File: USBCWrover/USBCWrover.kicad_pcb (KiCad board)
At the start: 2 copper layers, 21 parts, among them J1 USB_C_Receptacle_USB2.0, Q1 Q_NMOS_GSD, Q2 Q_NMOS_GSD, SW1 SW_Push, SW2 SW_Push, U1 CH340C, U2 CP2104, U3 AMS1117-3.3

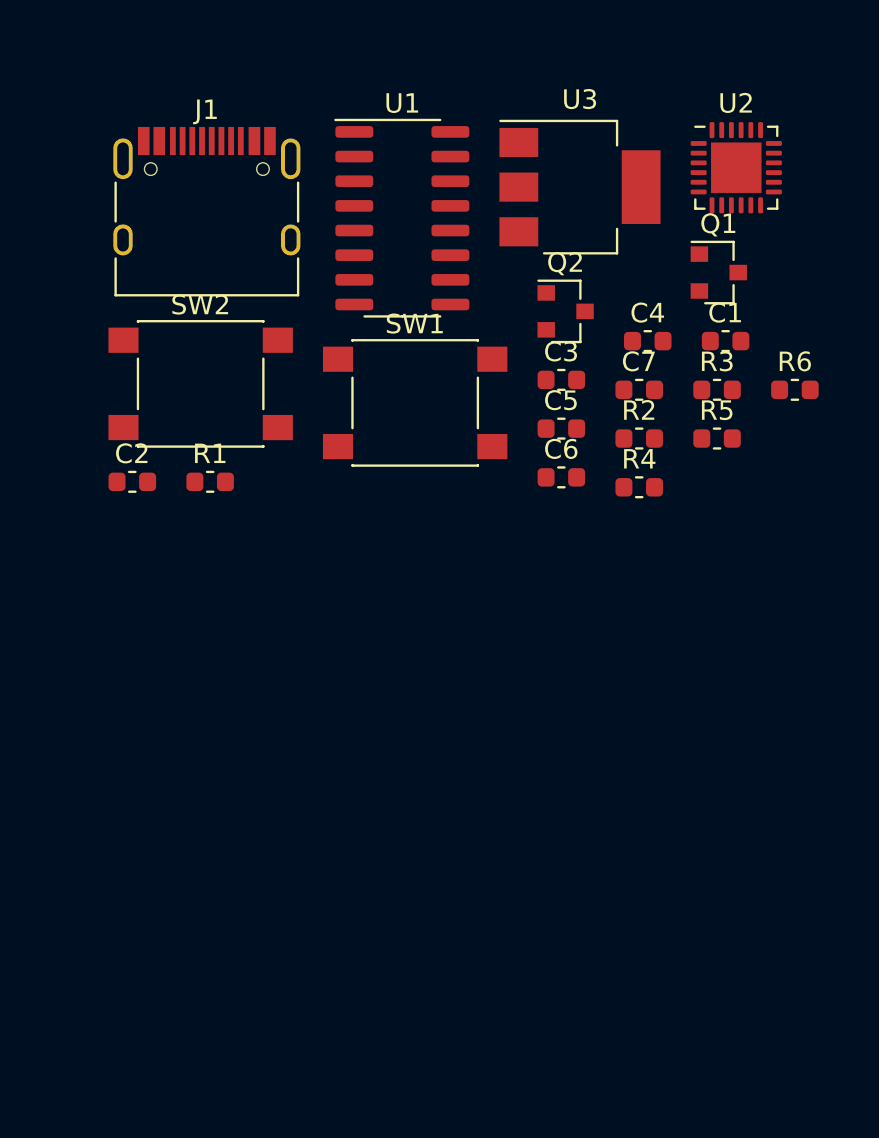
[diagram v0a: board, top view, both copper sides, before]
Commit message: routing done, but not pretty
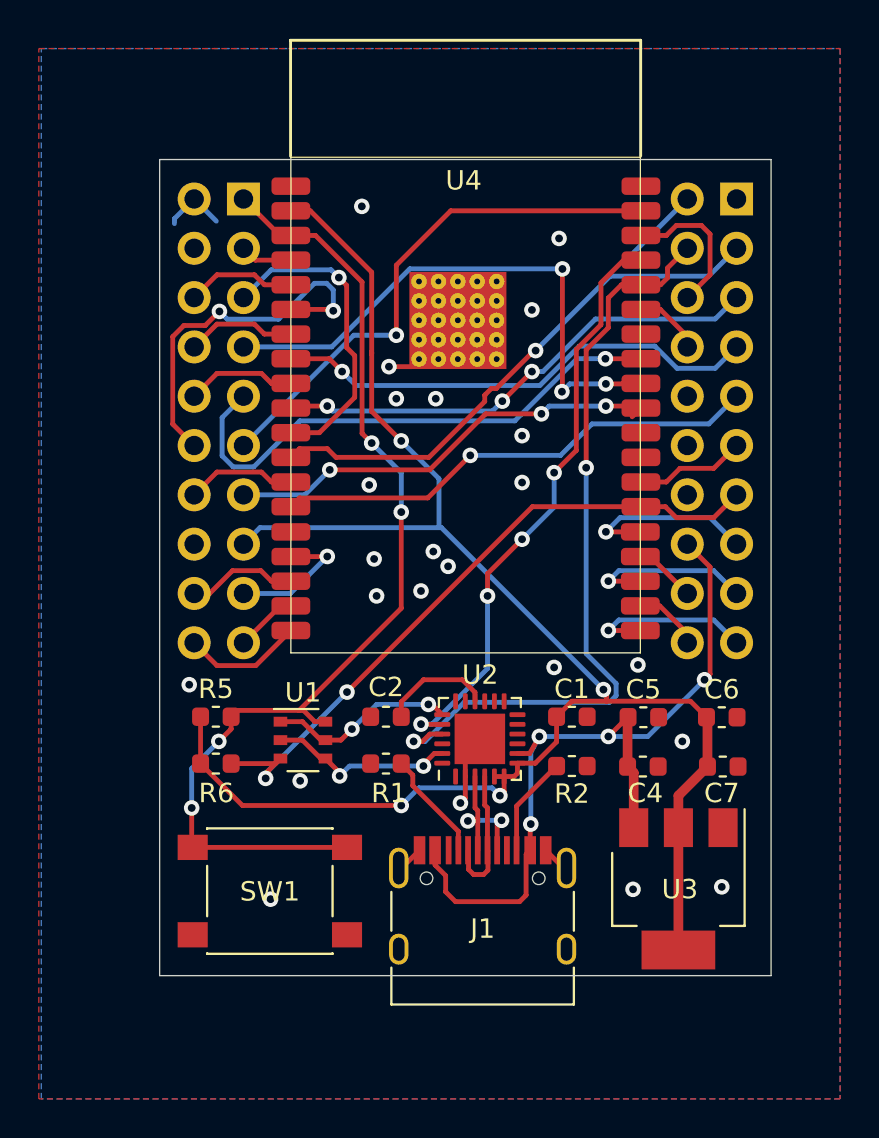
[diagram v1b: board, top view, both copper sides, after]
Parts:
- removed C3: 100nF, Capacitor_SMD:C_0603_1608Metric
- removed Q1, Q2: Q_NMOS_GSD, Package_TO_SOT_SMD:SOT-23
- removed R3, R4: 10k, Resistor_SMD:R_0603_1608Metric
- removed SW2: SW_Push, Button_Switch_SMD:SW_Push_1P1T_NO_6x6mm_H9.5mm
- added J2: Conn_02x10_Odd_Even, Connector_PinHeader_2.54mm:PinHeader_2x10_P2.54mm_Vertical, B.Cu at (154.9, 106.7)
- added J3: Conn_02x10_Odd_Even, Connector_PinHeader_2.54mm:PinHeader_2x10_P2.54mm_Vertical, B.Cu at (129.5, 106.7)
- added U4: ESP32-WROVER, esp32-wrover:ESP32-WROVER, F.Cu at (141.0, 105.1)
- U1: value CH340C -> UMH3N; footprint Package_SO:SOIC-16_3.9x9.9mm_P1.27mm -> Package_SO:TSOP-6_1.65x3.05mm_P0.95mm
- moved J1 39.2 mm to (141.9, 144.3)
- moved U3 36.5 mm to (151.9, 142.2), turned to 270 degrees
- moved R6 35.5 mm to (128.1, 135.8)
- moved U2 32.3 mm to (141.7, 134.5), turned to 90 degrees
- moved R5 29.5 mm to (128.1, 133.3)
- moved U1 27.4 mm to (132.6, 134.6)
- moved SW1 26.2 mm to (130.9, 142.3)
- moved C4 21.9 mm to (150.1, 135.9)
- moved C1 20.9 mm to (146.5, 133.3)
- moved C7 19.9 mm to (154.2, 135.9)
- moved C2 17.8 mm to (136.9, 133.3), turned to 180 degrees
- moved R2 17.2 mm to (146.5, 135.9), turned to 180 degrees
- moved R1 17.1 mm to (136.9, 135.8)
- moved C5 15.5 mm to (150.1, 133.4)
- moved C6 14.9 mm to (154.2, 133.4)
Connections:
- U1 pad 1: GND -> SER_RTS
- U1 pad 2: ESP_RXD -> SER_DTR
- U1 pad 3: ESP_TXD -> ESP_FLS
- U1 pad 4: Net-(U1-Pad4) -> SER_DTR
- U1 pad 5: USB_D+ -> SER_RTS
- U1 pad 6: USB_D- -> ESP_RST
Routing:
- net +3V3: track 0.00 -> 90.0 mm, vias 0 -> 4
- net ESP_RST: track 0.00 -> 53.7 mm, vias 0 -> 4
- net +5V: track 0.00 -> 41.4 mm, vias 0 -> 4
- net ESP_RXD: track 0.00 -> 40.1 mm, vias 0 -> 2
- net ESP_TXD: track 0.00 -> 35.0 mm, vias 0 -> 4
- net ESP_FLS: track 0.00 -> 34.9 mm, vias 0 -> 2
- net IO18: track 0.00 -> 29.6 mm, vias 0 -> 3
- net IO27: track 0.00 -> 28.0 mm, vias 0 -> 1
- net IO19: track 0.00 -> 27.6 mm, vias 0 -> 1
- net IO23: track 0.00 -> 27.6 mm, vias 0 -> 1
- net IO25: track 0.00 -> 25.5 mm, vias 0 -> 3
- net IO12: track 0.00 -> 25.3 mm, vias 0 -> 1
- net IO32: track 0.00 -> 25.3 mm, vias 0 -> 1
- net IO5: track 0.00 -> 23.0 mm, vias 0 -> 3
- net GND: track 0.00 -> 20.1 mm, vias 0 -> 23
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- added copper zone on B.Cu, net GND
- added copper zone on F.Cu, net GND
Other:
- board outline added: 31.5 x 42 mm
- net class Default: clearance 0.2 -> 0.127
- rule trace_clearance: 0.2 -> 0.127
